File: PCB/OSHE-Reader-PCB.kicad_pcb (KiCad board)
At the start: 2 copper layers, 8.7 x 4.4 mm, 73 parts, among them J1 USB_C_Receptacle_PowerOnly_24P, J2 112L-TDA0, J3 Conn_01x24_MountingPin, Q1 PNP, Q2 Si1308EDL, SW1 SW_Push, SW2 SW_Push, SW3 SW_Push, SW4 SW_Push, SW5 SW_Push, U1 BQ2057CSNTR, U2 IRF7326D2TRPBF, U3 TPS5432DDA

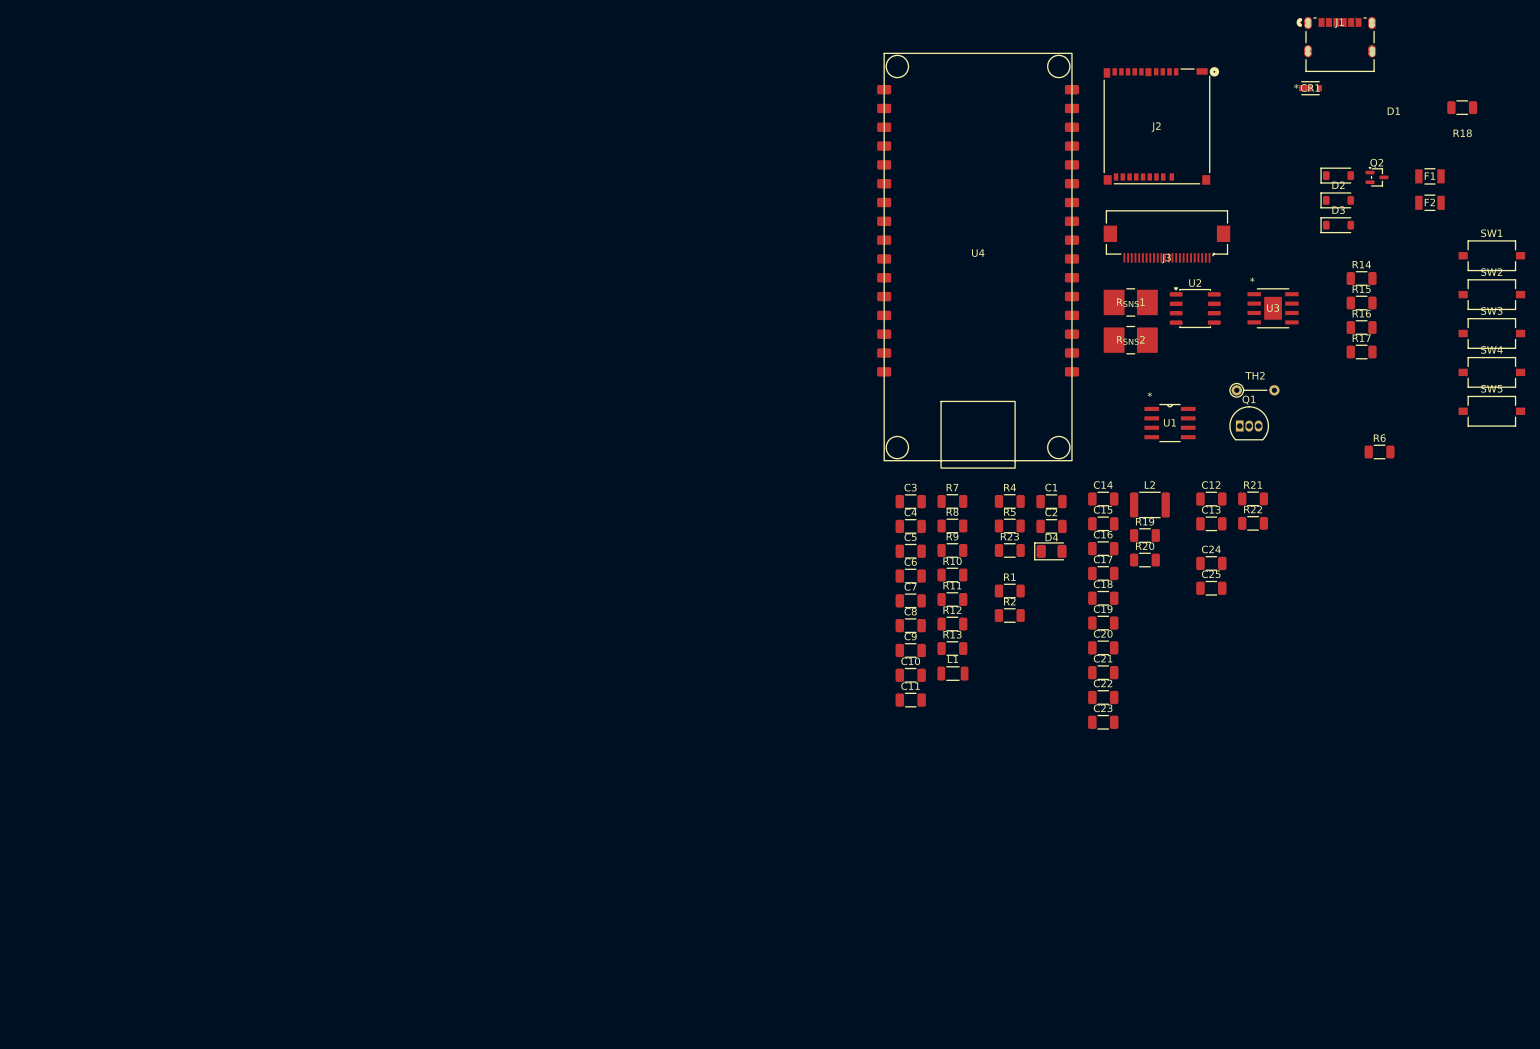
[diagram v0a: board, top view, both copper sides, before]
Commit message: PCB Work
Fiddled with PCB :/
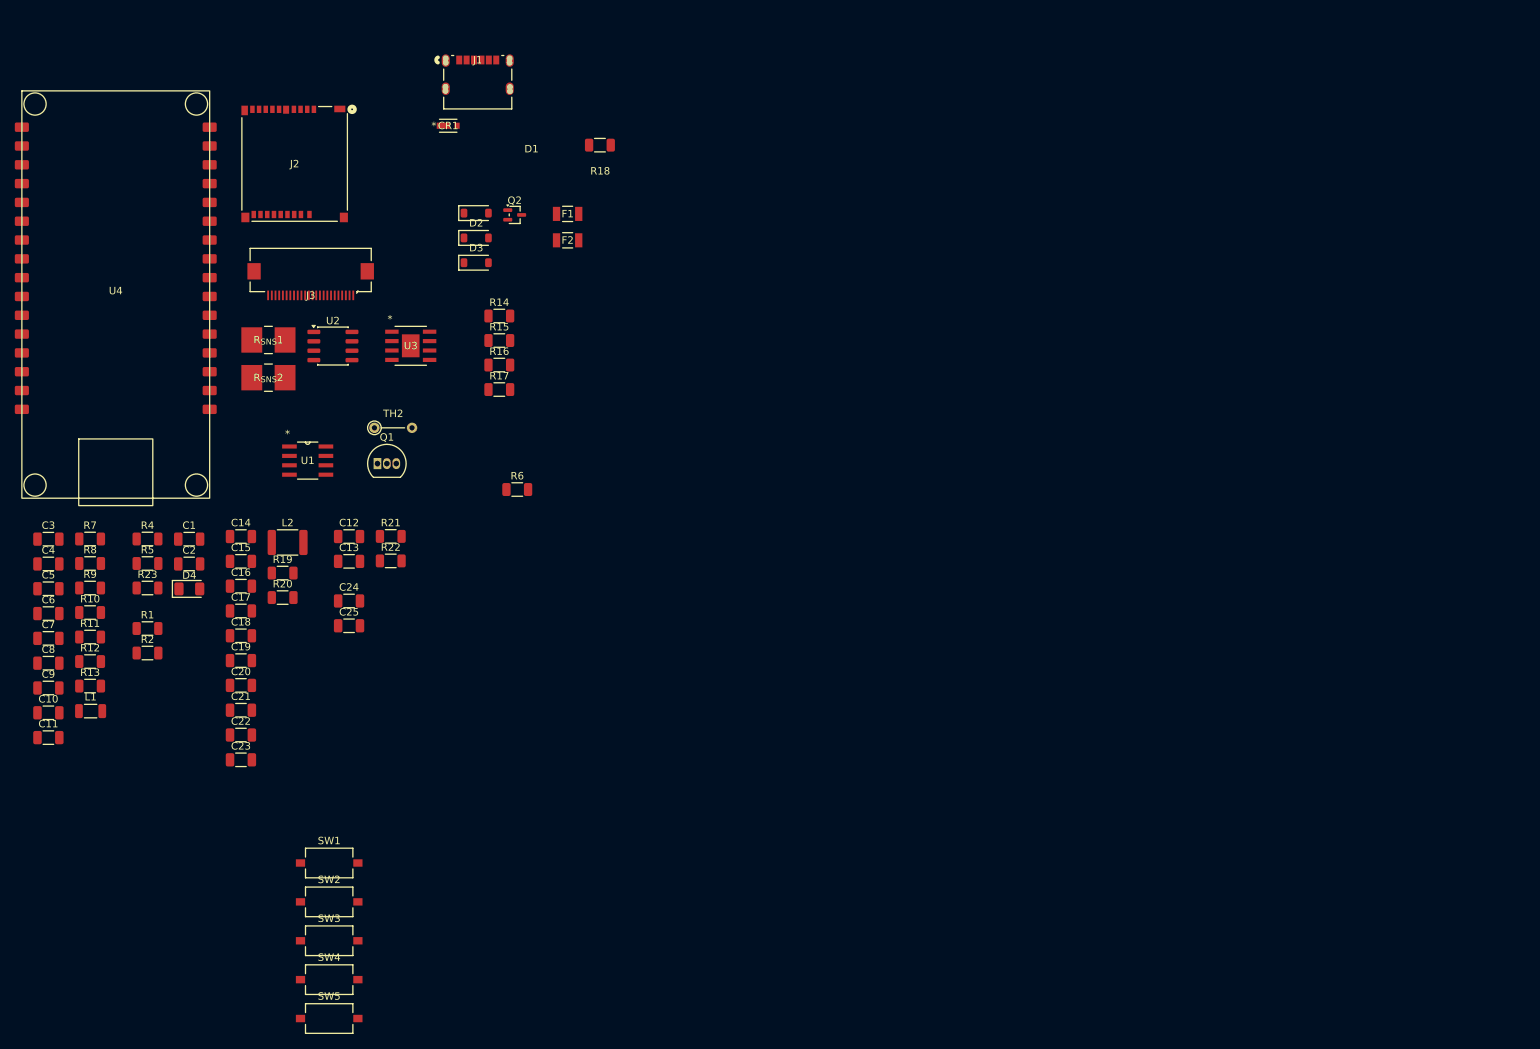
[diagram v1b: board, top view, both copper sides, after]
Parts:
- moved SW1 177.1 mm to (-49.5, 130.5)
- moved SW2 177.1 mm to (-49.5, 135.8)
- moved SW3 177.1 mm to (-49.5, 141.0)
- moved SW4 177.1 mm to (-49.5, 146.2)
- moved SW5 177.1 mm to (-49.5, 151.5)
- moved C10 116.6 mm to (-87.4, 110.2)
- moved C11 116.6 mm to (-87.4, 113.6)
- moved C12 116.6 mm to (-46.8, 86.4)
- moved C13 116.6 mm to (-46.8, 89.8)
- moved C14 116.6 mm to (-61.4, 86.4)
- moved C15 116.6 mm to (-61.4, 89.8)
- moved C16 116.6 mm to (-61.4, 93.1)
- moved C17 116.6 mm to (-61.4, 96.5)
- moved C18 116.6 mm to (-61.4, 99.8)
- moved C19 116.6 mm to (-61.4, 103.2)
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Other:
- copper layers 2 -> 4
